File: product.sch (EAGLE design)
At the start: 41 parts, among them IC1 MCP1703CB, Q2 16MHz, U1 ATSHA204-TSU, U2 USB, U3 DISPLAY, U4 TPD4S014_DSQ_10

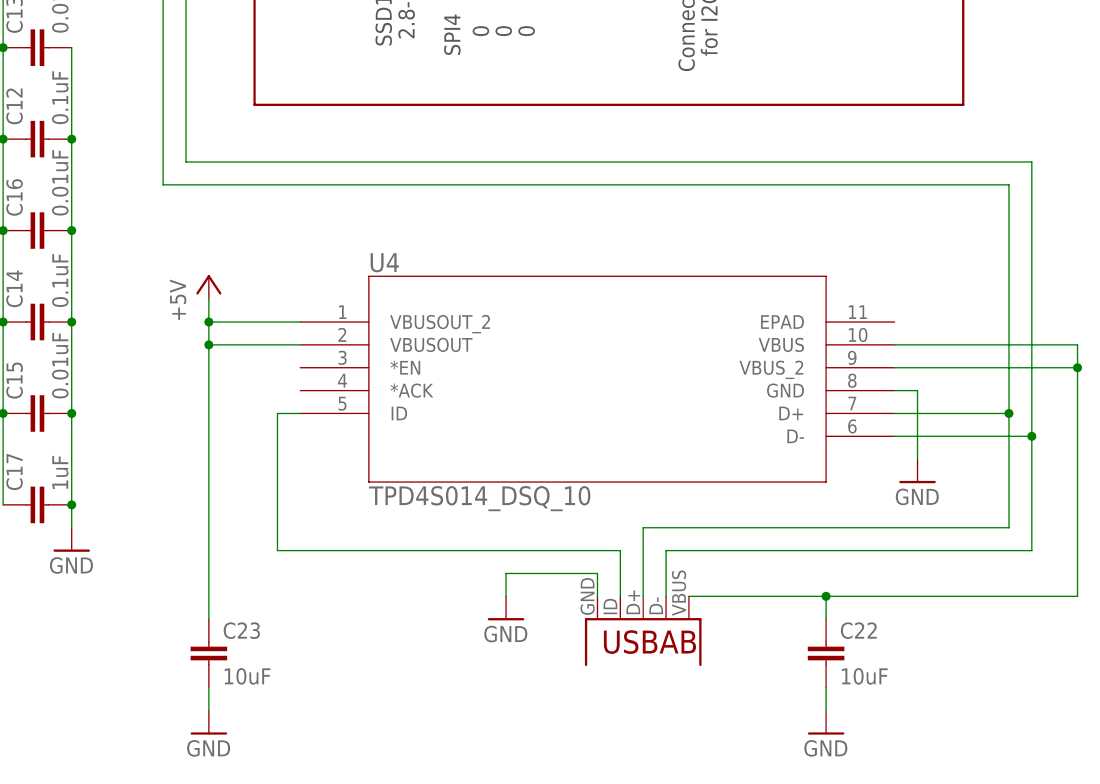
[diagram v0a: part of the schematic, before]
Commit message: work in progress
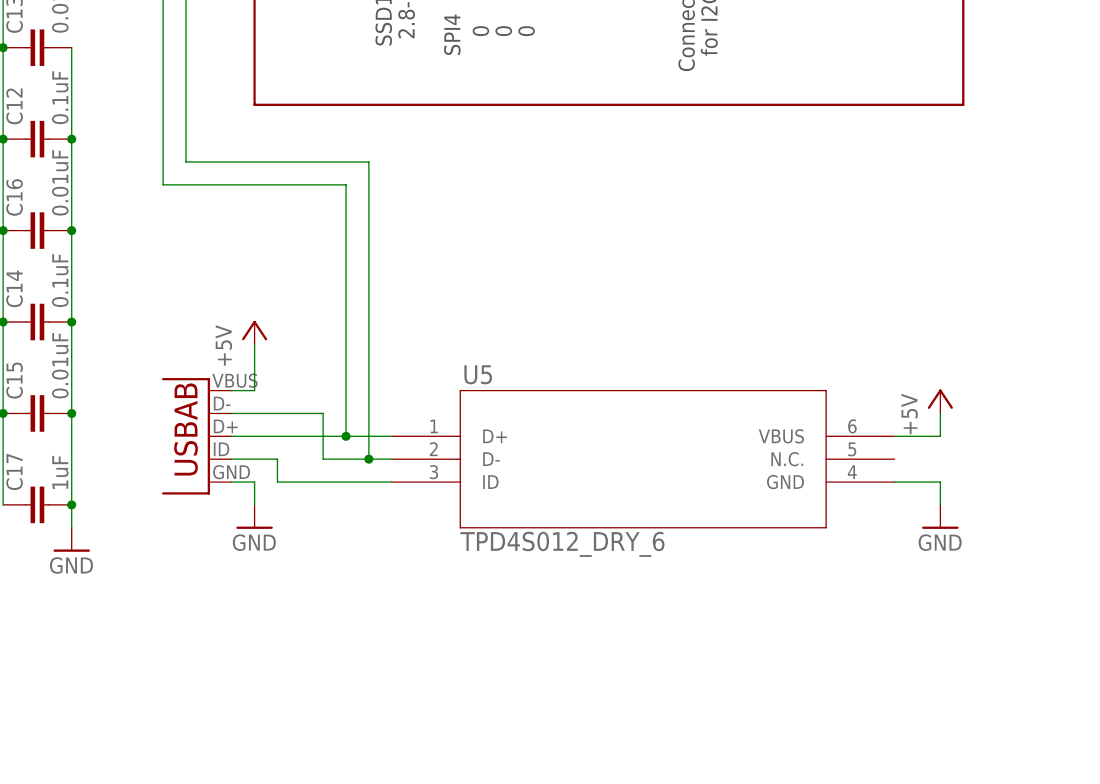
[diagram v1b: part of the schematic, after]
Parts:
- removed C22, C23: 10uF, SparkFun-Passives:CAP0402-CAP
- removed U4: TPD4S014_DSQ_10, imported:TPD4S014_DSQ_10
- added U5: TPD4S012_DRY_6, imported:TPD4S012_DRY_6
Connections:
- removed net N$7: C22.1, U2.VBUS, U4.VBUS, U4.VBUS_2
- net +5V: now also U2.VBUS, U5.VBUS; no longer C23.1, U4.VBUSOUT, U4.VBUSOUT_2
- net GND: now also U5.GND; no longer C22.2, C23.2, U4.GND
- net N$3: now also U5.ID; no longer U4.ID
- net USB_D_N: now also U5.D-; no longer U4.D-
- net USB_D_P: now also U5.D+; no longer U4.D+
